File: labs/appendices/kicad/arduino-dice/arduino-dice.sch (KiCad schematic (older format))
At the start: 10 parts, among them IC1 ATMEGA328P-P, P1 CONN_01X02, SW1 SW_PUSH, Y1 16 MHz

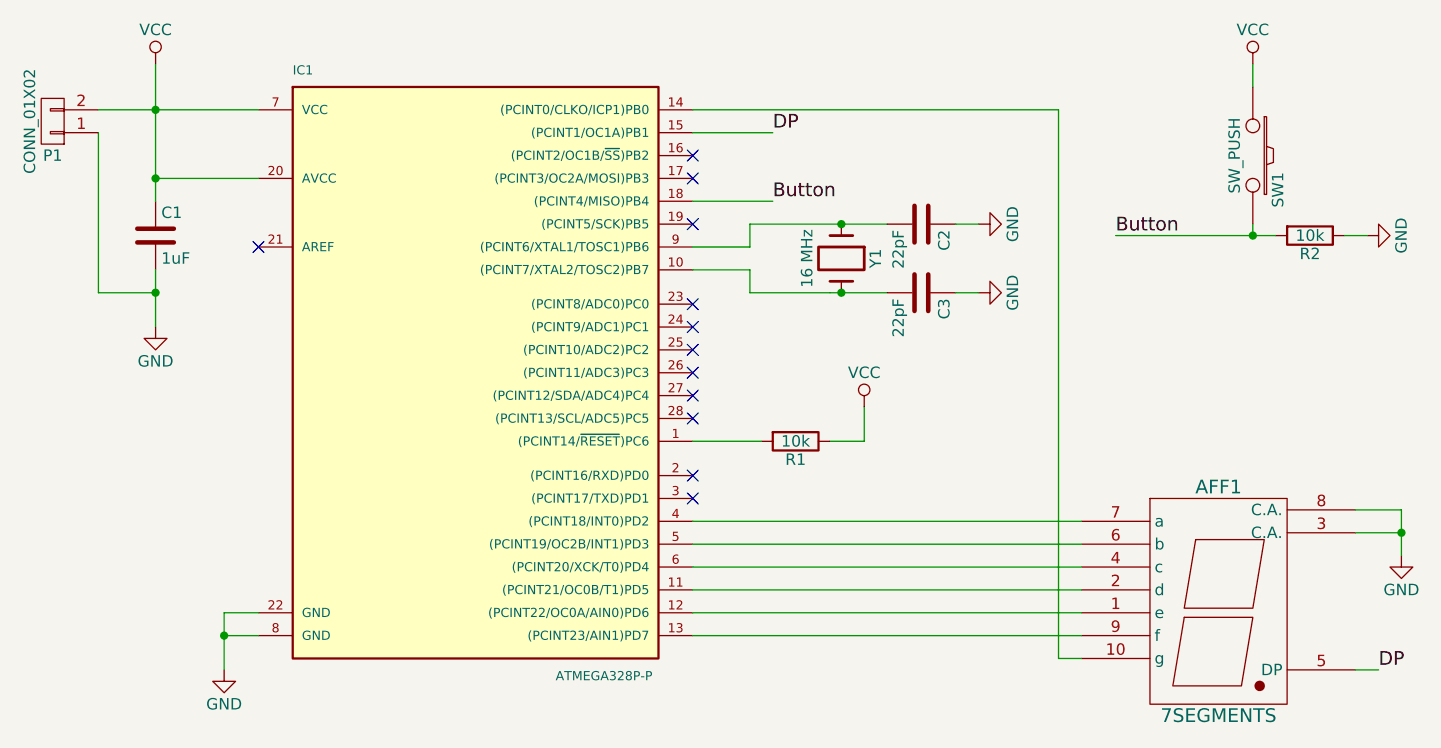
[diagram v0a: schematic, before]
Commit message: update
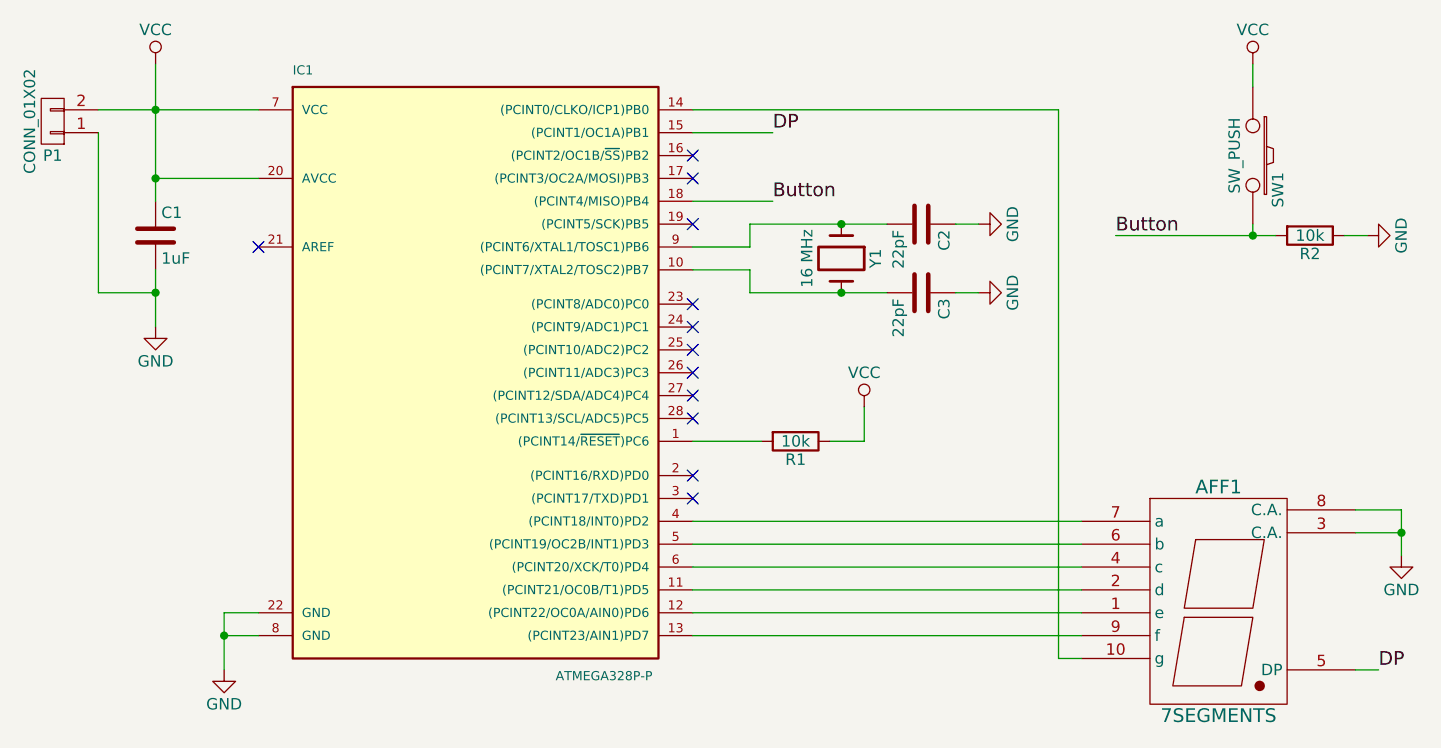
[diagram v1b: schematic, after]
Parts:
- AFF1: footprint (none) -> arduino-dice-footprints:7segment-hdsp-313e
- C1, C2, C3, R1, R2: footprint (none) -> arduino-dice-footprints:smd_0603
- IC1: footprint (none) -> arduino-dice-footprints:atmega328p-pu
- P1: footprint (none) -> Pin_Headers:Pin_Header_Straight_1x02
- SW1: footprint (none) -> arduino-dice-footprints:sw_push_b3f_1000
- Y1: footprint (none) -> arduino-dice-footprints:crystal_hc49us
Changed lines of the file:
@@
 F 0 "IC1" H 2550 4700 40  0000 L BNN
 F 1 "ATMEGA328P-P" H 3700 2050 40  0000 L BNN
-F 2 "" H 3300 3450 30  0000 C CIN
+F 2 "arduino-dice-footprints:atmega328p-pu" H 3300 3450 30  0001 C CIN
 F 3 "" H 3300 3450 60  0000 C CNN
 	1    3300 3450
@@
 F 0 "R2" V 7080 2900 50  0000 C CNN
 F 1 "10k" V 7000 2900 50  0000 C CNN
-F 2 "" V 6930 2900 30  0000 C CNN
+F 2 "arduino-dice-footprints:smd_0603" V 6930 2900 30  0001 C CNN
 F 3 "" H 7000 2900 30  0000 C CNN
 	1    7000 2900
@@
 F 0 "AFF1" H 6600 5100 60  0000 C CNN
 F 1 "7SEGMENTS" H 6600 4100 60  0000 C CNN
-F 2 "" H 6600 4550 60  0000 C CNN
+F 2 "arduino-dice-footprints:7segment-hdsp-313e" H 6600 4550 60  0001 C CNN
 F 3 "" H 6600 4550 60  0000 C CNN
 	1    6600 4550
@@
 F 0 "R1" V 4830 3800 50  0000 C CNN
 F 1 "10k" V 4750 3800 50  0000 C CNN
-F 2 "" V 4680 3800 30  0000 C CNN
+F 2 "arduino-dice-footprints:smd_0603" V 4680 3800 30  0001 C CNN
 F 3 "" H 4750 3800 30  0000 C CNN
 	1    4750 3800
@@
 F 0 "Y1" H 4950 3150 50  0000 C CNN
 F 1 "16 MHz" H 4950 2850 50  0000 C CNN
-F 2 "" H 4950 3000 60  0000 C CNN
+F 2 "arduino-dice-footprints:crystal_hc49us" H 4950 3000 60  0001 C CNN
 F 3 "" H 4950 3000 60  0000 C CNN
 	1    4950 3000
@@
 F 0 "C2" H 5325 2950 50  0000 L CNN
 F 1 "22pF" H 5325 2750 50  0000 L CNN
-F 2 "" H 5338 2700 30  0000 C CNN
+F 2 "arduino-dice-footprints:smd_0603" H 5338 2700 30  0001 C CNN
 F 3 "" H 5300 2850 60  0000 C CNN
 	1    5300 2850
@@
 F 0 "C3" H 5325 3250 50  0000 L CNN
 F 1 "22pF" H 5325 3050 50  0000 L CNN
-F 2 "" H 5338 3000 30  0000 C CNN
+F 2 "arduino-dice-footprints:smd_0603" H 5338 3000 30  0001 C CNN
 F 3 "" H 5300 3150 60  0000 C CNN
 	1    5300 3150
@@
 F 0 "SW1" H 6900 2660 50  0000 C CNN
 F 1 "SW_PUSH" H 6750 2470 50  0000 C CNN
-F 2 "" H 6750 2550 60  0000 C CNN
+F 2 "arduino-dice-footprints:sw_push_b3f_1000" H 6750 2550 60  0001 C CNN
 F 3 "" H 6750 2550 60  0000 C CNN
 	1    6750 2550
@@
 	4550 3050 4550 3150
 Wire Wire Line
-	4550 3150 4900 3150
-Wire Wire Line
-	4900 3150 5150 3150
+	4550 3150 5150 3150
 Wire Wire Line
 	4650 2750 4300 2750
 Wire Wire Line
-	6150 2900 6750 2900
-Wire Wire Line
-	6750 2900 6850 2900
+	6150 2900 6850 2900
 Wire Wire Line
 	6000 4650 4300 4650
@@
 F 0 "C1" H 1975 3000 50  0000 L CNN
 F 1 "1uF" H 1975 2800 50  0000 L CNN
-F 2 "" H 1988 2750 30  0000 C CNN
+F 2 "arduino-dice-footprints:smd_0603" H 1988 2750 30  0001 C CNN
 F 3 "" H 1950 2900 60  0000 C CNN
 	1    1950 2900
@@
 F 0 "P1" H 1500 2550 50  0000 C CNN
 F 1 "CONN_01X02" V 1600 2400 50  0000 C CNN
-F 2 "" H 1500 2400 60  0000 C CNN
+F 2 "Pin_Headers:Pin_Header_Straight_1x02" H 1500 2400 60  0001 C CNN
 F 3 "" H 1500 2400 60  0000 C CNN
 	1    1500 2400
@@
 $EndComp
 Wire Wire Line
-	1700 2350 1950 2350
-Wire Wire Line
-	1950 2350 2400 2350
+	1700 2350 2400 2350
 Wire Wire Line
 	1700 2450 1700 3150
@@
 	1700 3150 1950 3150
 Wire Wire Line
-	1950 3050 1950 3150
-Wire Wire Line
-	1950 3150 1950 3300
-Wire Wire Line
-	1950 2150 1950 2350
-Wire Wire Line
-	1950 2350 1950 2650
-Wire Wire Line
-	1950 2650 1950 2750
+	1950 3050 1950 3300
+Wire Wire Line
+	1950 2150 1950 2750
 Wire Wire Line
 	1950 2650 2400 2650
@@
 	2400 4650 2250 4650
 Wire Wire Line
-	2250 4550 2250 4650
-Wire Wire Line
-	2250 4650 2250 4800
+	2250 4550 2250 4800
 Wire Wire Line
 	2400 4550 2250 4550
@@
 	7200 4200 7400 4200
 Wire Wire Line
-	7400 4100 7400 4200
-Wire Wire Line
-	7400 4200 7400 4300
+	7400 4100 7400 4300
 Wire Wire Line
 	7200 4100 7400 4100
